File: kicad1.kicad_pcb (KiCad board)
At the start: 2 copper layers, 100 x 80 mm, 44 parts

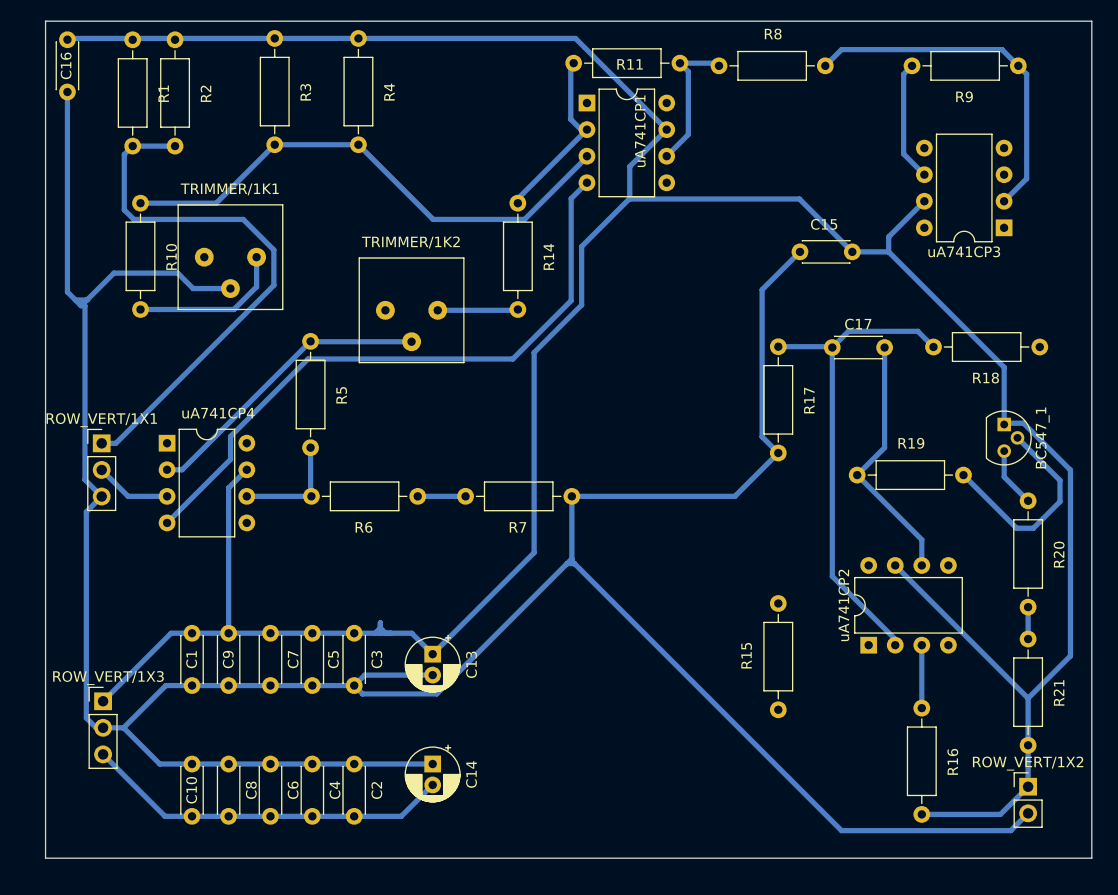
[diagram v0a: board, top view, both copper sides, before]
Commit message: done
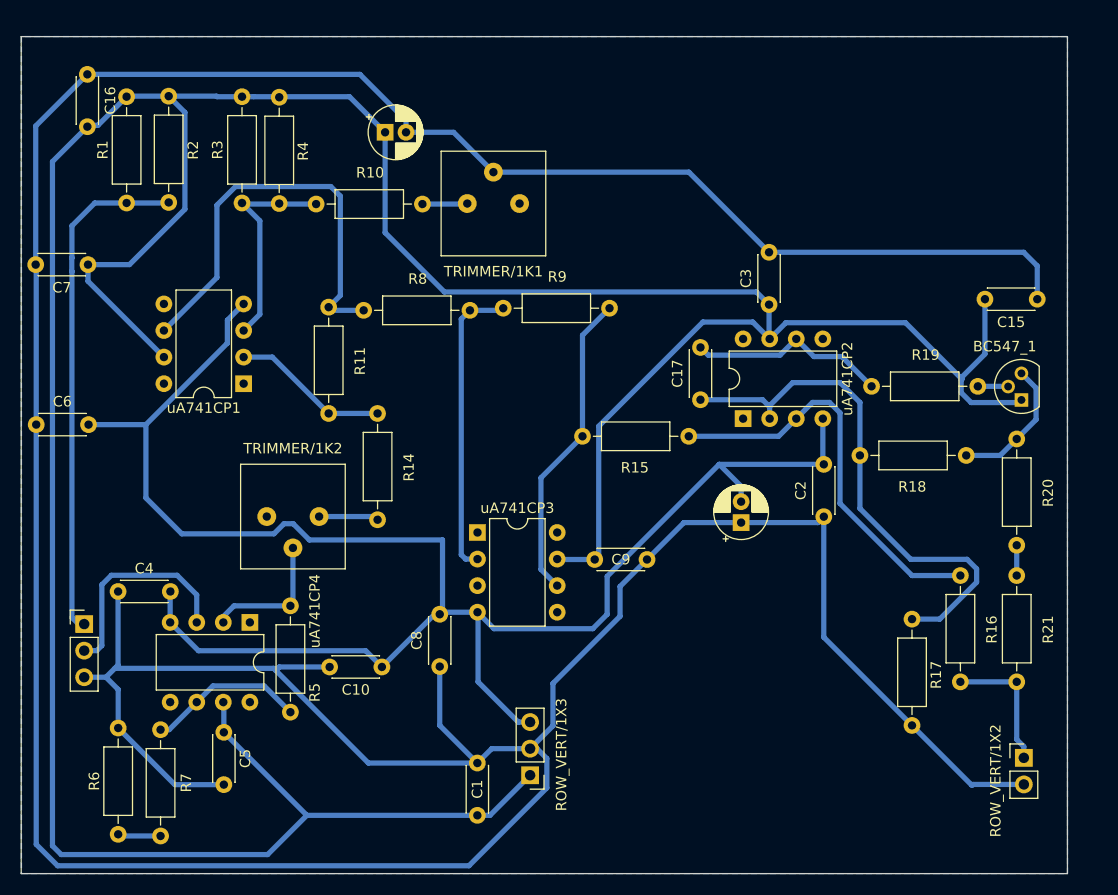
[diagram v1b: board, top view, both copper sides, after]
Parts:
- moved uA741CP3 58.1 mm to (132.3, 93.4), turned to 0 degrees
- moved C2 50.7 mm to (165.4, 91.9), turned to 90 degrees
- moved C3 50.6 mm to (160.2, 71.6), turned to 90 degrees
- moved C13 50.1 mm to (123.5, 55.1), turned to 0 degrees
- moved R7 47.0 mm to (97.9, 117.2), turned to 90 degrees
- moved R9 45.3 mm to (139.9, 71.9), turned to 180 degrees
- moved uA741CP1 42.4 mm to (109.9, 79.1), turned to 180 degrees
- moved ROW_VERT/1X3 41.4 mm to (137.3, 116.6), turned to 180 degrees
- moved R8 41.2 mm to (126.6, 72.1)
- moved R11 40.2 mm to (118.1, 77.0), turned to 90 degrees
- moved C6 39.4 mm to (90.1, 83.1), turned to 0 degrees
- moved C7 39.3 mm to (95.1, 67.8), turned to 180 degrees
- moved C14 37.4 mm to (157.5, 92.4), turned to 90 degrees
- moved C9 35.7 mm to (143.5, 96.0), turned to 0 degrees
- moved R6 33.5 mm to (102.0, 117.2), turned to -90 degrees
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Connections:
- R16 pad 1: +15V -> Net-(ROW_VERT/1X2-Pin_1)
- R21 pad 1: +15V -> Net-(ROW_VERT/1X2-Pin_1)
- ROW_VERT/1X2 pad 1: +15V -> Net-(ROW_VERT/1X2-Pin_1)
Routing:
- net GND: track 277.1 -> 402.3 mm
- net -15V: track 95.8 -> 166.1 mm
- net Net-(uA741CP2-+): track 6.24 -> 39.2 mm
- net Net-(uA741CP1-+): track 50.5 -> 20.8 mm
- net Net-(R11-Pad2): track 13.9 -> 41.5 mm
- net +15V: track 299.7 -> 326.6 mm
- net Net-(R15-Pad1): track 11.8 -> 29.9 mm
- net Net-(BC547_1-B): track 20.2 -> 2.90 mm
- net Net-(uA741CP4--): track 28.5 -> 13.0 mm
- net Net-(ROW_VERT/1X1-Pin_2): track 7.29 -> 20.6 mm
- net Net-(ROW_VERT/1X2-Pin_1): track 0.00 -> 12.9 mm
- net Net-(R10-Pad1): track 14.8 -> 4.31 mm
- net Net-(BC547_1-E): track 5.70 -> 13.1 mm
- net Net-(C17-Pad2): track 24.6 -> 19.2 mm
- net Net-(uA741CP3--): track 33.9 -> 28.7 mm
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- added copper zone on B.Cu, net +15V
